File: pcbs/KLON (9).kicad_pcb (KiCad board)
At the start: 2 copper layers, 159.6 x 117.7 mm, 91 parts

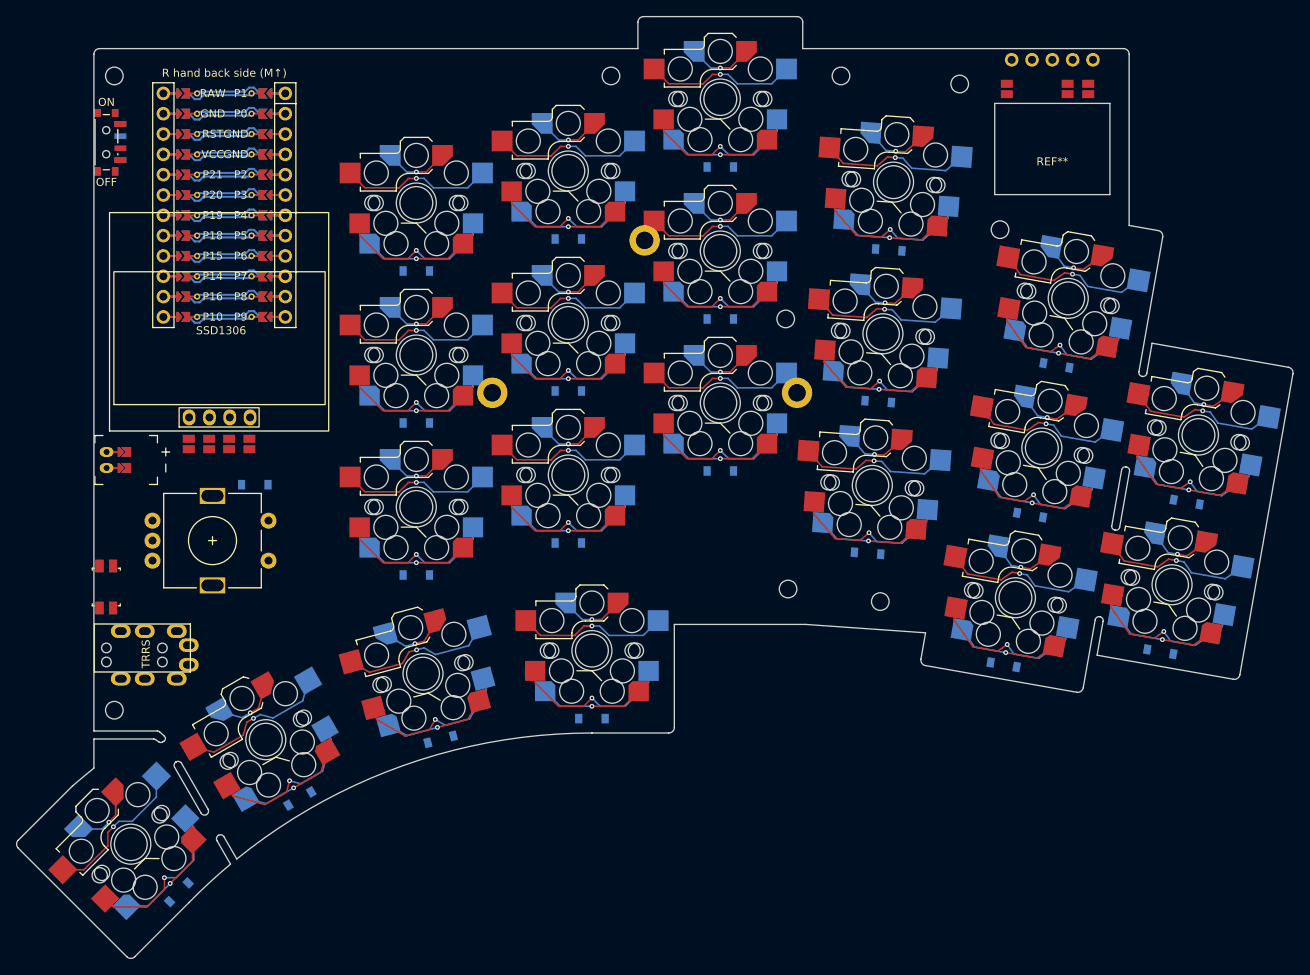
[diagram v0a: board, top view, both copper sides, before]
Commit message: pcb updates
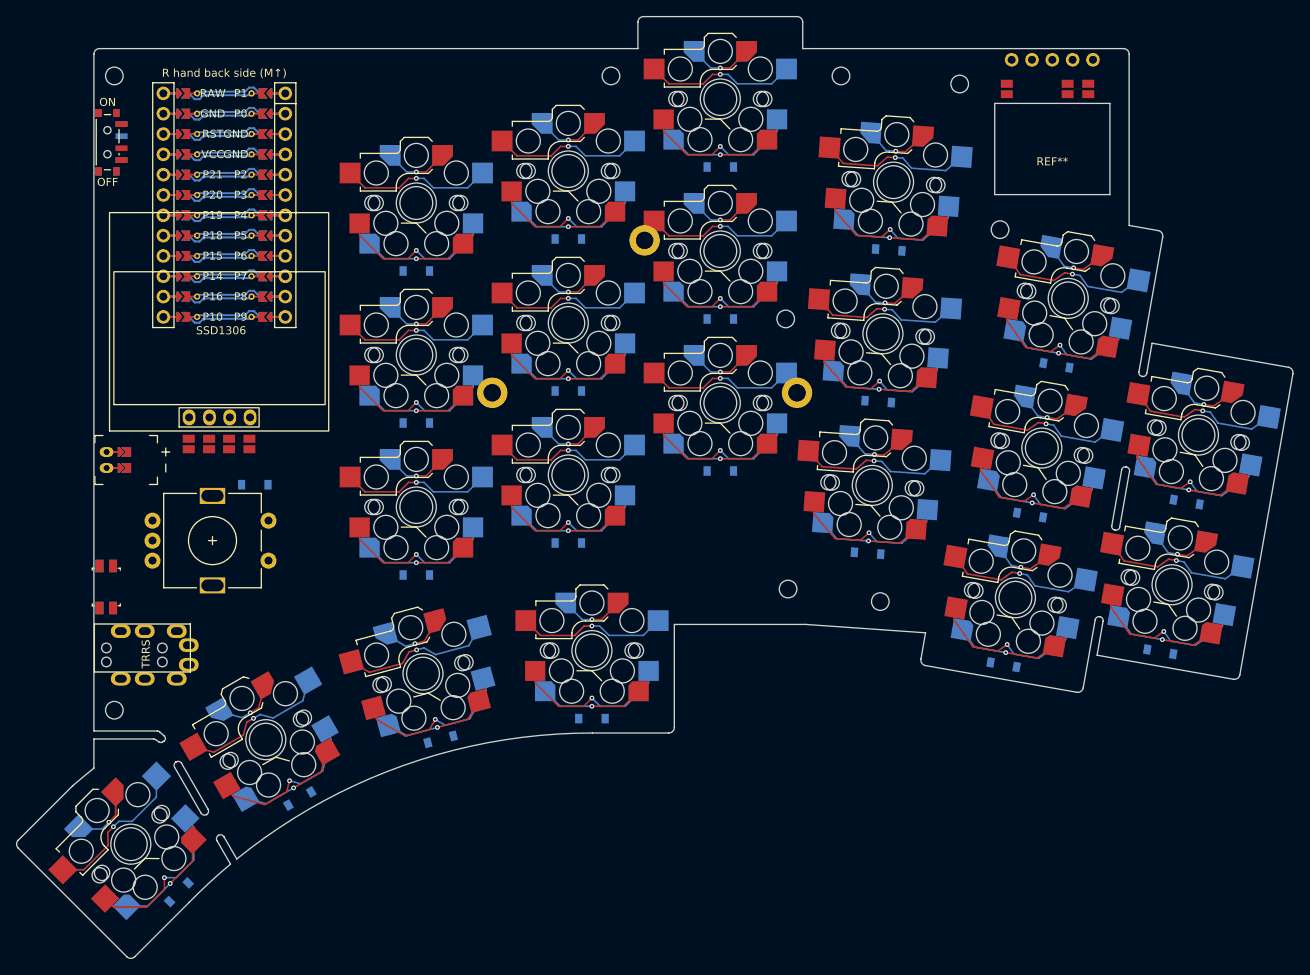
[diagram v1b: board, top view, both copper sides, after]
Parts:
- removed XX1: , Pimoroni Haptic Buzz DRV2605L Driver
- removed XX2: , RotaryEncoder_Alps_EC11E-Switch_Vertical_H20mm-keebio_modified
- removed XX3: , SSD1306_128x64OLED
- removed XX4: , MJ-4PP-9
- added J1: MJ-4PP-9, MJ-4PP-9, F.Cu at (129.8, 167.6)
- added REF**: Pimoroni Haptic Buzz DRV2605L Driver, Pimoroni Haptic Buzz DRV2605L Driver, F.Cu at (249.5, 104.5)
- added SSD1306: SSD1306_128x64OLED, SSD1306_128x64OLED, F.Cu at (145.6, 128.2)
- added SW25: Rotary_Encoder_Switch, RotaryEncoder_Alps_EC11E-Switch_Vertical_H20mm-keebio_modified, F.Cu at (144.5, 154.2)
- moved PWR1 0.15 mm to (131.4, 104.4)
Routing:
- net (no net): track 337.7 -> 0.00 mm
- net P4: track 75.4 -> 124.7 mm
- net P3: track 75.4 -> 124.7 mm
- net P6: track 56.6 -> 96.0 mm
- net P7: track 56.6 -> 96.0 mm
- net P5: track 56.6 -> 96.0 mm
- net P8: track 37.7 -> 67.2 mm
- net GND: track 0.00 -> 29.5 mm
- net P10: track 18.9 -> 38.5 mm
- net P16: track 18.9 -> 38.5 mm
- net pinky_home: track 42.2 -> 32.3 mm
- net ring_bottom: track 42.2 -> 32.3 mm
- net ring_home: track 42.2 -> 32.3 mm
- net ring_top: track 42.2 -> 32.3 mm
- net 4_r0: track 42.2 -> 32.3 mm
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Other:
- outline, holes or cut-outs redrawn
